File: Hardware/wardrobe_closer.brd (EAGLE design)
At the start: 27.9 x 32.7 mm, 9 parts, among them U1 ATTINY25-20SHR

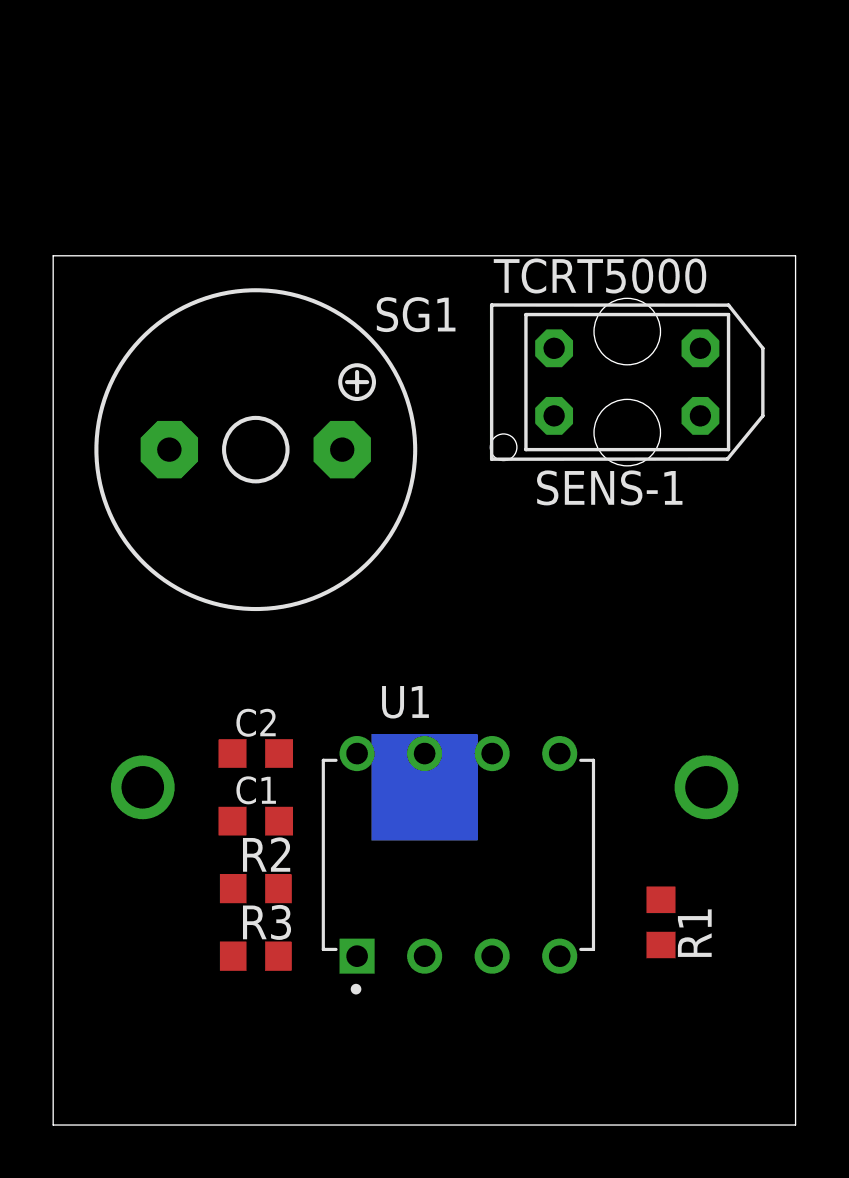
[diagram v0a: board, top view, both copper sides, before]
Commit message: Update design
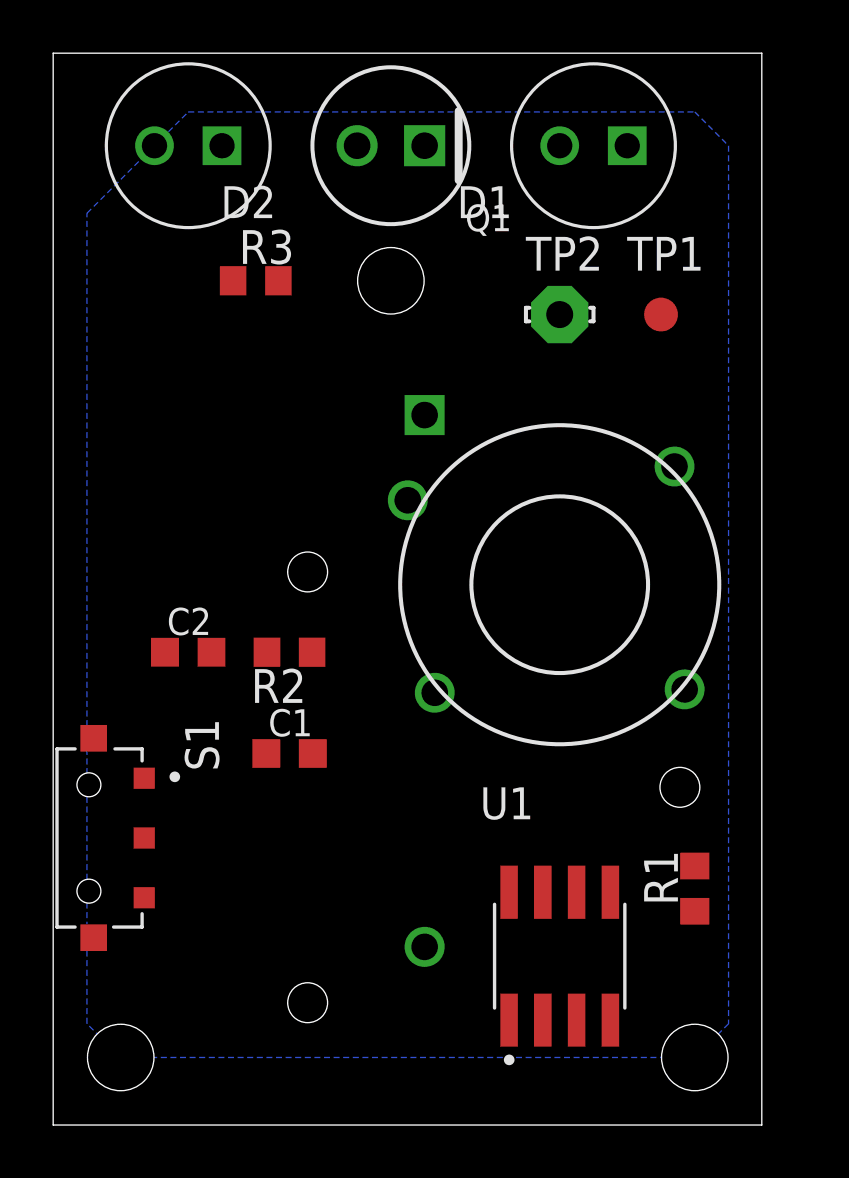
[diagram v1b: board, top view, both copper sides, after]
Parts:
- removed SENS-1: TCRT5000, qfm-trx1-24g:5000
- removed SG1: F/QMBIII, buzzer:F/QMBIII
- added D1, D2: WP7113SGD, LED:RADIAL_5MM
- added Q1: EVERLIGHT_PT334-6BEVERLIGHT_PT334-6B_0_0, Everlight - PT334-6B:EVERLIGHT_PT334-6B_0
- added S1: JS102000SAQN, Switch:JS102000SAQN
- added TP1: TPB1,27, BeagleBone_Blue_R3:B1,27
- added TP2: LSP10, solpad:LSP10
- BT1: value 79523211 -> 79528211; device Battery Holder:79523211 -> Battery Holder:79528211
- R3: value (none) -> 100
- U1: device Microcontroller:PDIP-8 -> Microcontroller:SOIC-8
- moved R3 25.4 mm to (7.62, 31.8)
- moved R2 8.98 mm to (8.89, 17.8), turned to 180 degrees
- moved U1 5.39 mm to (19.1, 6.35)
- moved C2 4.58 mm to (5.08, 17.8)
- moved C1 2.84 mm to (8.89, 14.0)
- moved R1 1.80 mm to (24.1, 8.89), turned to 90 degrees
- turned BT1 to 270 degrees
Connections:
- removed net N$3: R3.1, SG1.+
- new net BEEP: TP1.TP, U1.3
- new net LED: R3.2, U1.6
- new net N$7: D2.A, R3.1
- net DET: now also Q1.2, U1.2; no longer SENS-1.P$1, U1.5
- net EMT: now also U1.7; no longer U1.6
- net GND: now also BT1.1, D1.C, D2.C, Q1.1, TP2.MP; no longer BT1.P1, BT1.P2, SENS-1.P$2, SENS-1.P$4, SG1.-
- net N$1: now also D1.A; no longer SENS-1.P$3
- net N$2: now also BT1.2, S1.1; no longer R3.2, U1.3
- net VCC: now also S1.2; no longer BT1.N
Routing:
- added copper zone on layer 16, net GND
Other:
- board size 27.9 x 32.7 mm -> 26.6 x 40.3 mm
